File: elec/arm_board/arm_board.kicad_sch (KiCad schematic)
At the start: 37 parts, among them J1 PinHeader, J12 B2B-XH-A(LF)(SN), J16 B4B-ZR(LF)(SN), J2 PinHeader, J3 B6B-ZR, J4 Fan motor, SW1 B3U-3000P, U1 NA219AIDR, U12 OKL-T/6-W12N-C, U17 FT231XQ-R, U2 TB67H450, U3 ATmega328P-AU, X1 CSTCE16M0V53-R0

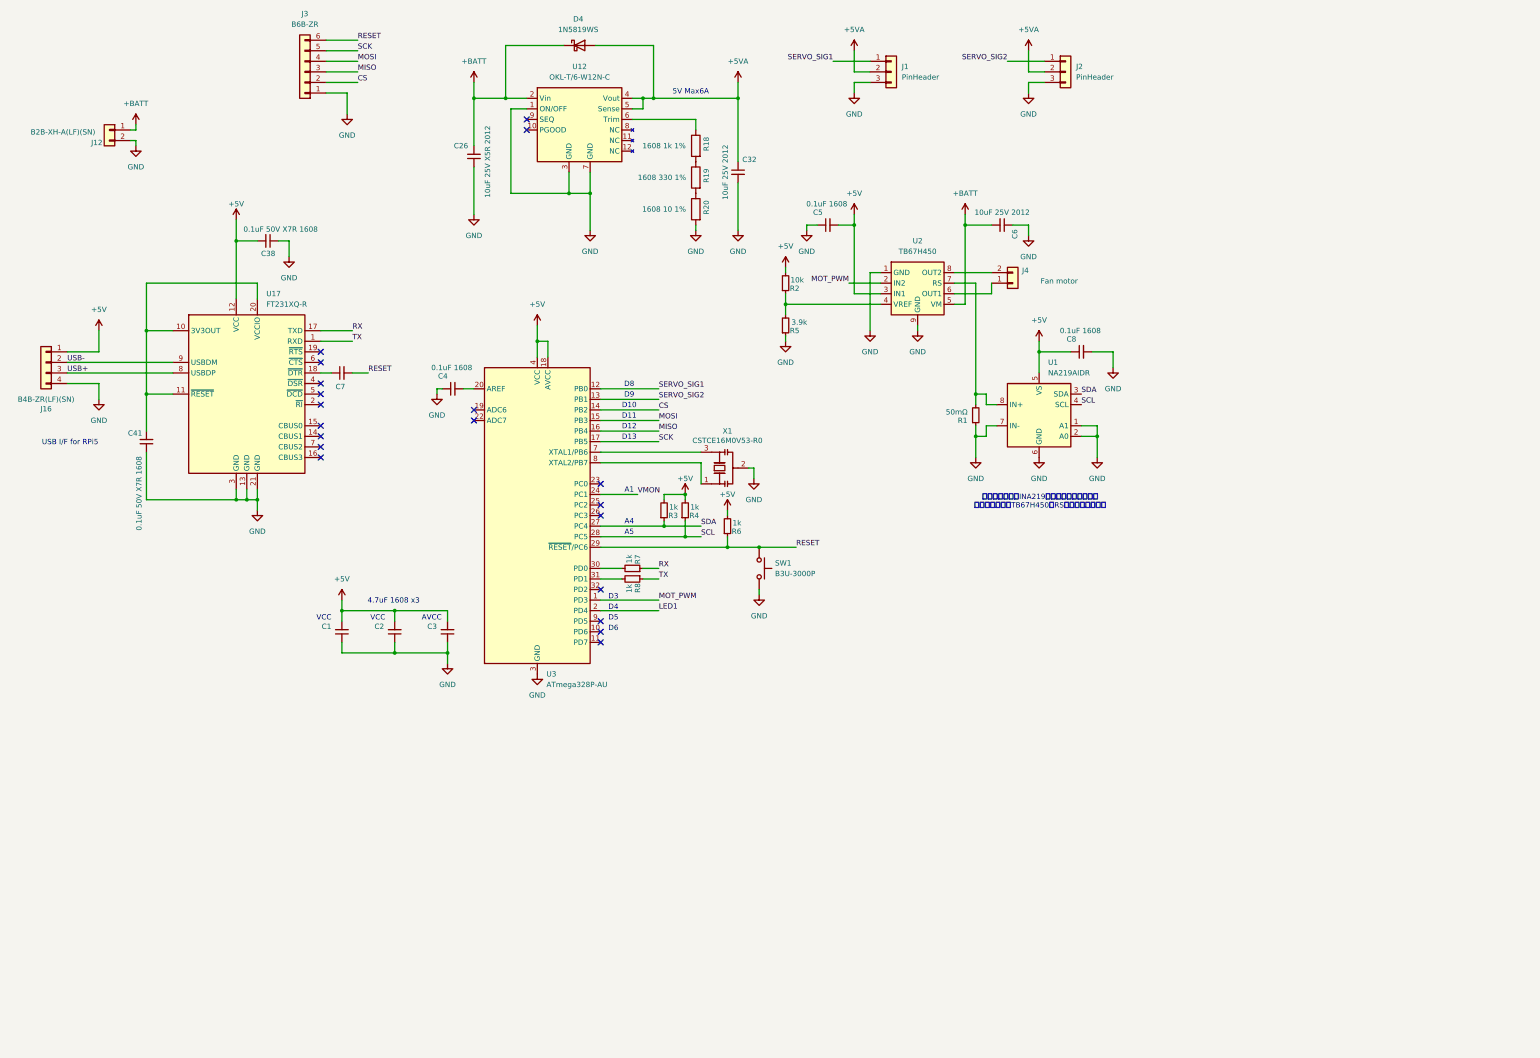
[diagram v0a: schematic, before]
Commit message: ARMボード発注
Signed-off-by: Kazuki Iida <elkel53930@gmail.com>
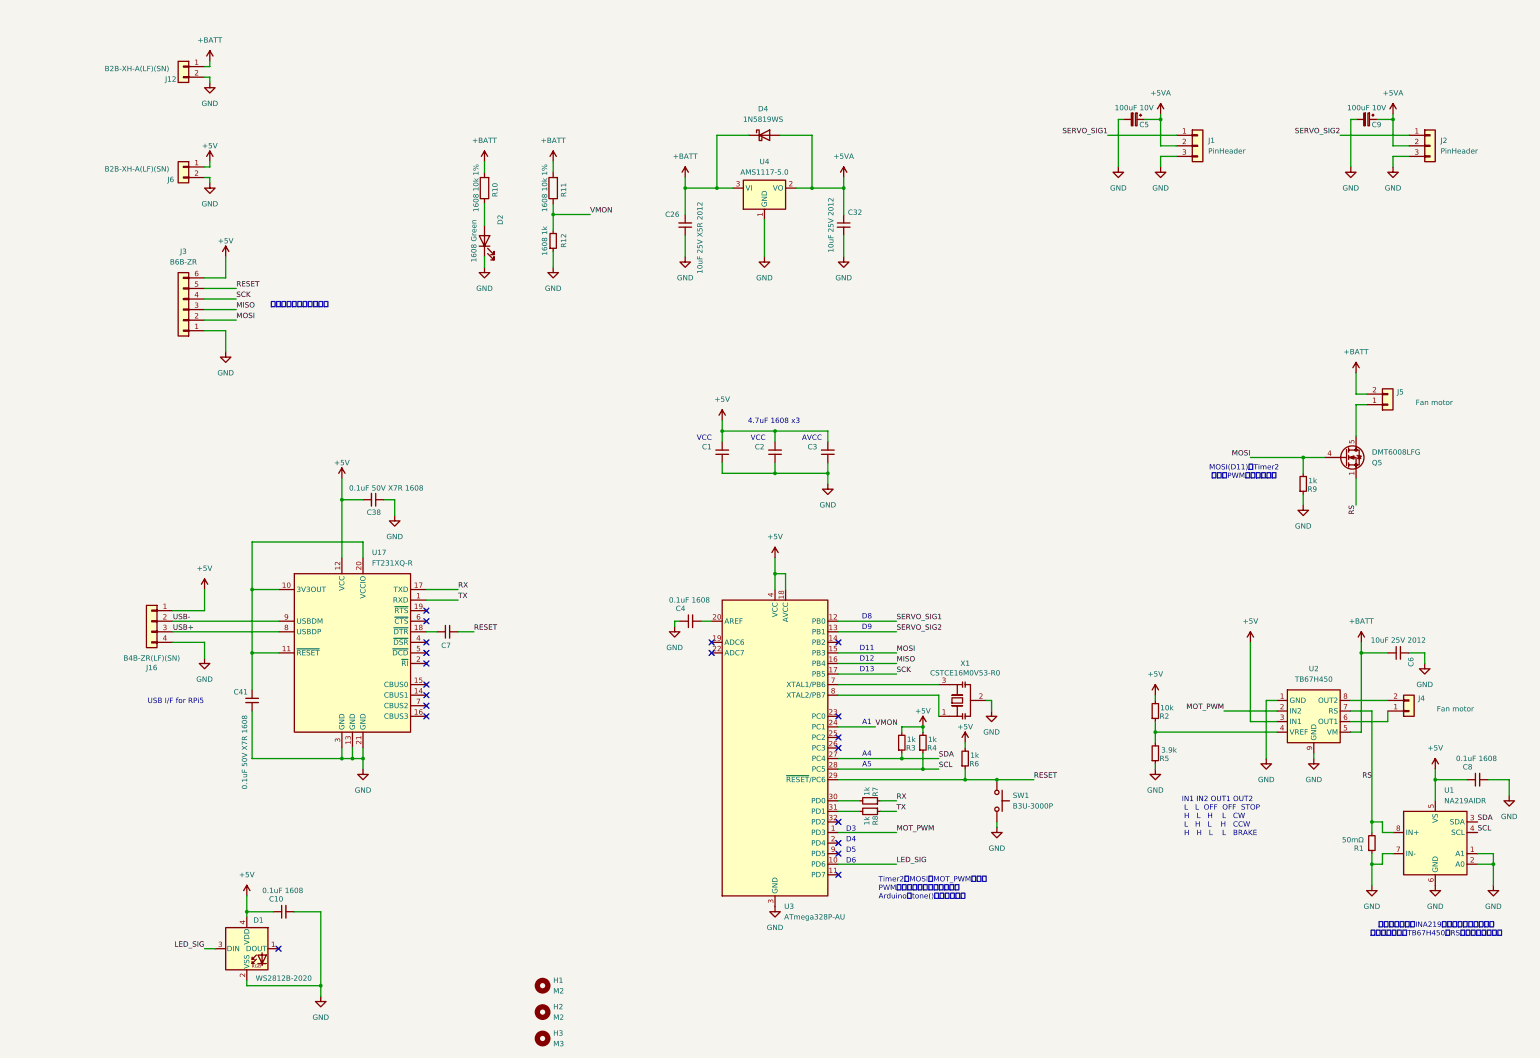
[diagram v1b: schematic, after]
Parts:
- removed C5: CC0603KRX7R9BB104, Capacitor_SMD:C_0603_1608Metric, symbol Device:C_Small
- removed R18: 0603WAF1001T5E, Resistor_SMD:R_0603_1608Metric, symbol Device:R
- removed R19: 0603WAF3300T5E, Resistor_SMD:R_0603_1608Metric, symbol Device:R
- removed R20: 0603WAF100JT5E, Resistor_SMD:R_0603_1608Metric, symbol Device:R
- removed U12: OKL-T/6-W12N-C, Library:OKL-T&slash_6-W12N-C_MUR, symbol micromouse-twilight:OKL-T/6-W12N-C
- added C10: CC0603KRX7R9BB104, Capacitor_SMD:C_0603_1608Metric, symbol Device:C_Small
- added C5, C9: RVT1A101M0505, Capacitor_SMD:CP_Elec_5x5.4, symbol Device:C_Polarized_Small
- added D1: WS2812B-2020, LED_SMD:LED_WS2812B-2020_PLCC4_2.0x2.0mm, symbol LED:WS2812B-2020
- added D2: D-060306G1/SS2/G1, LED_SMD:LED_0603_1608Metric, symbol Device:LED
- added H1, H2: M2, MountingHole:MountingHole_2.2mm_M2, symbol Mechanical:MountingHole
- added H3: M3, MountingHole:MountingHole_3.2mm_M3, symbol Mechanical:MountingHole
- added J5: Fan motor, Connector_PinHeader_2.54mm:PinHeader_1x02_P2.54mm_Vertical, symbol Connector_Generic:Conn_01x02
- added J6: B2B-XH-A(LF)(SN), Connector_JST:JST_XH_B2B-XH-AM_1x02_P2.50mm_Vertical, symbol Connector_Generic:Conn_01x02
- added Q5: DMT6008LFG, Package_SON:Diodes_PowerDI3333-8, symbol Transistor_FET:DMT6008LFG
- added R10, R11: 0603WAF1002T5E, Resistor_SMD:R_0603_1608Metric, symbol Device:R
- added R12, R9: 0603WAF1001T5E, Resistor_SMD:R_0603_1608Metric, symbol Device:R_Small
- added U4: AMS1117-5.0, Package_TO_SOT_SMD:SOT-223-3_TabPin2, symbol Regulator_Linear:AMS1117-5.0
- X1: footprint Ceralock:CSTCE -> Crystal:Resonator_SMD_Murata_CSTxExxV-3Pin_3.0x1.1mm
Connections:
- net +5V: now also J3.6 (Pin_6), C10.1, D1.4 (VDD), J6.1 (Pin_1)
- net +5VA: now also C5.1, C9.1, U4.2 (VO)
- net +BATT: now also J5.2 (Pin_2), R10.2, R11.2, U4.3 (VI)
- net GND: now also C10.2, C5.2, C9.2, D1.2 (VSS), D2.1 (K), J6.2 (Pin_2), R12.1, R9.1, U4.1 (GND)
- net MOSI: now also J3.2 (Pin_2), Q5.4 (G), R9.2; no longer J3.4 (Pin_4)
- net RESET: now also J3.5 (Pin_5); no longer J3.6 (Pin_6)
- net SCK: now also J3.4 (Pin_4); no longer J3.5 (Pin_5)
- net VMON: now also R11.1, R12.2
- net LED_SIG: now reaches U3.10 (PD6)
- net LED_SIG: now also D1.3 (DIN)
- net RS: now reaches R1.2, U1.8 (IN+), U2.7 (RS)
- net RS: now also Q5.1 (S), Q5.2 (S), Q5.3 (S)
- net CS: no longer names the net of U3.14 (PB2)
- net CS: no longer J3.2 (Pin_2)
- net LED1: no longer names the net of U3.2 (PD4)
- new net: J5.1 (Pin_1), Q5.5 (D)
- new net: D2.2 (A), R10.1
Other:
- note added: "IN1 IN2 OUT1 OUT2 L L OFF OFF STOP H L H L CW L H L H CCW H H L L BRAKE"
- note added: "MOSI(D11)はTimer2 によるPWM信号と兼用。"
- note added: "Timer2はMOSIとMOT_PWMからの PWM信号生成に使用するため、 Arduinoのtone()は使用不可。"
- note added: "ブートローダー書込み用"
- note removed: "5V Max6A"
- note removed: "D10"
- moved on the sheet: C1, C2, C26, C3, C32, C38, C4, C41, C6, C7, C8, D4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
